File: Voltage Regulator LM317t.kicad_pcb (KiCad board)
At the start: 2 copper layers, 55.8 x 28 mm, 15 parts, among them J1 IN, J2 OUT, U1 LM317_TO-220

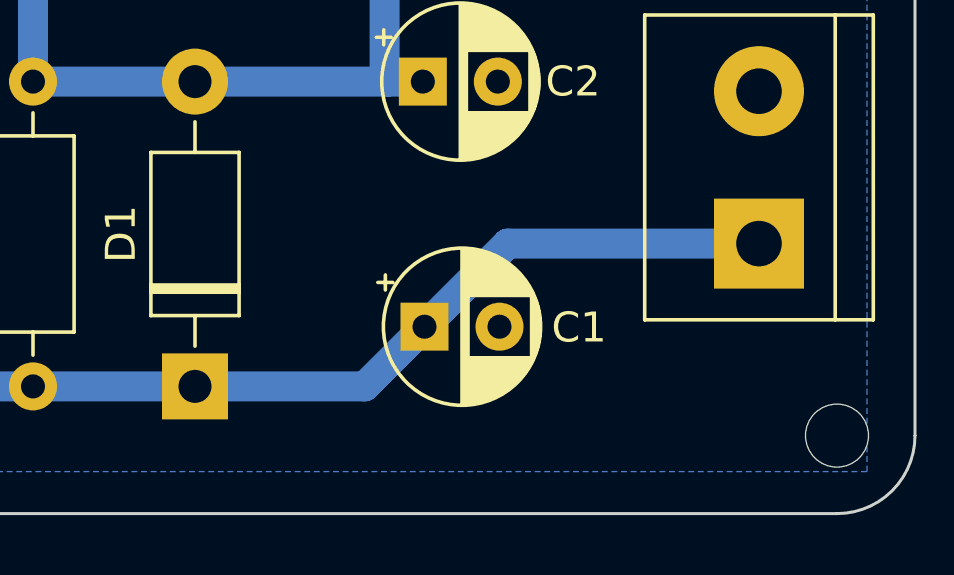
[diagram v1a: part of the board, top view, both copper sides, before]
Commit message: interactive bom
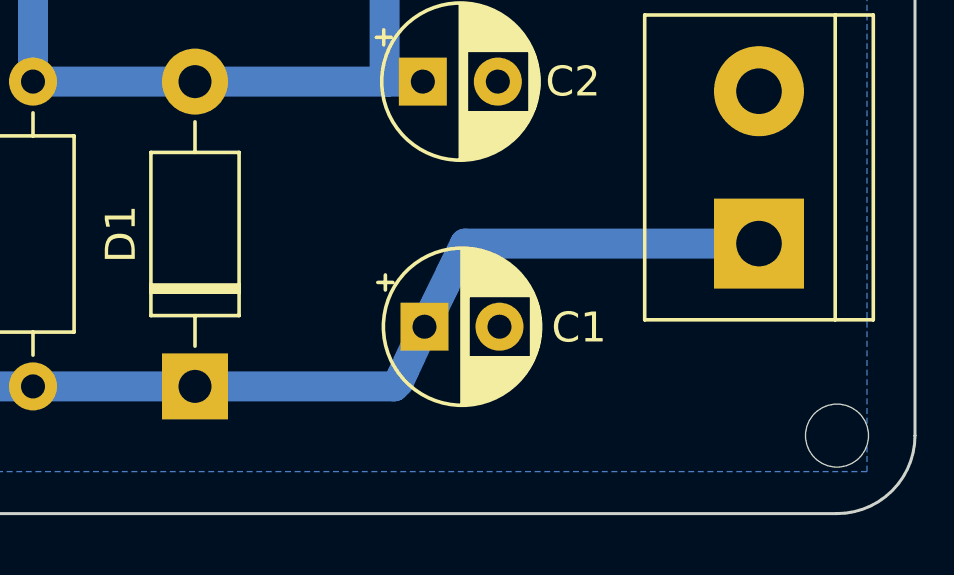
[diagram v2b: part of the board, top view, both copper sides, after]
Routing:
- net /OUTPUT: track 50.2 -> 51.2 mm
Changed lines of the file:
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@@
   )
   (paper "A4")
+  (title_block
+    (title "Voltage Regulator LM317T")
+    (date "2023-08-16")
+    (rev "1.0.0")
+  )
   (layers
-    (0 "F.Cu" signal)
-    (31 "B.Cu" signal)
+    (0 "F.Cu" power)
+    (31 "B.Cu" mixed)
     (32 "B.Adhes" user "B.Adhesive")
     (33 "F.Adhes" user "F.Adhesive")
@@
       (outputformat 1)
       (mirror false)
-      (drillshape 1)
+      (drillshape 0)
       (scaleselection 1)
-      (outputdirectory "")
+      (outputdirectory "./")
     )
   )
@@
     (property "ki_keywords" "mounting hole")
     (attr exclude_from_pos_files exclude_from_bom)
-    (fp_text reference "H1" (at -35.2 13.2) (layer "F.SilkS") hide
+    (fp_text reference "H1" (at 0 -4.2) (layer "F.SilkS") hide
         (effects (font (size 1 1) (thickness 0.15)))
     )
@@
         (effects (font (size 1 1) (thickness 0.15)))
     )
-    (fp_text user "${REFERENCE}" (at 2.54 -4.27) (layer "F.Fab")
+    (fp_text user "${REFERENCE}" (at 9 -0.05) (layer "F.Fab")
         (effects (font (size 1 1) (thickness 0.15)))
     )
@@
     (pad "3" thru_hole oval (at 5.08 0 180) (size 1.905 2) (drill 1.1) (layers "*.Cu" "*.Mask")
       (net 4 "/INPUT") (pinfunction "VI") (pintype "power_in"))
-    (model "${KIPRJMOD}/packages3D/TO-220-3_Vertical.wrl"
+    (model "${KICAD6_3DMODEL_DIR}/Package_TO_SOT_THT.3dshapes/TO-220-3_Vertical.wrl"
       (offset (xyz 0 0 0))
       (scale (xyz 1 1 1))
@@
         (effects (font (size 1 1) (thickness 0.15)))
     )
-    (fp_text value "Logo_Open_Hardware_Small" (at 0.75 0) (layer "B.Fab") hide
-        (effects (font (size 1 1) (thickness 0.15)) (justify mirror))
+    (fp_text value "Logo_Open_Hardware_Small" (at 0.75 0) (layer "F.SilkS") hide
+        (effects (font (size 1 1) (thickness 0.15)))
     )
     (fp_poly
@@
     (effects (font (size 1.5 1.5) (thickness 0.3) bold) (justify left bottom mirror))
   )
-  (segment (start 167.4 112.8) (end 159.02 112.8) (width 1) (layer "B.Cu") (net 1))
+  (dimension (type aligned) (layer "Dwgs.User")
+    (pts (xy 116.8 119.2) (xy 172.6 119.2))
+    (height 7.999999)
+    (gr_text "55.8000 mm" (at 144.7 126.049999) (layer "Dwgs.User")
+      (effects (font (size 1 1) (thickness 0.15)))
+    )
+    (format (prefix "") (suffix "") (units 3) (units_format 1) (precision 4))
+    (style (thickness 0.15) (arrow_length 1.27) (text_position_mode 0) (extension_height 0.58642) (extension_offset 0.5) keep_text_aligned)
+  )
+  (dimension (type aligned) (layer "Dwgs.User")
+    (pts (xy 170 121.8) (xy 170 93.8))
+    (height 11)
+    (gr_text "28.0000 mm" (at 179.85 107.8 90) (layer "Dwgs.User")
+      (effects (font (size 1 1) (thickness 0.15)))
+    )
+    (format (prefix "") (suffix "") (units 3) (units_format 1) (precision 4))
+    (style (thickness 0.15) (arrow_length 1.27) (text_position_mode 0) (extension_height 0.58642) (extension_offset 0.5) keep_text_aligned)
+  )
+  (dimension (type radial) (layer "Dwgs.User")
+    (pts (xy 119.4 119.2) (xy 117.561522 121.038478))
+    (leader_length 3.81)
+    (gr_text "R 2.6000 mm" (at 102.167445 123.732555) (layer "Dwgs.User")
+      (effects (font (size 1.5 1.5) (thickness 0.3)))
+    )
+    (format (prefix "R ") (suffix "") (units 3) (units_format 1) (precision 4))
+    (style (thickness 0.2) (arrow_length 1.27) (text_position_mode 0) (extension_offset 0.5) keep_text_aligned)
+  )
+  (segment (start 157.6 112.8) (end 156.25 115.57) (width 1) (layer "B.Cu") (net 1))
   (segment (start 140.6 117.56) (end 143.2 117.56) (width 1) (layer "B.Cu") (net 1))
   (segment (start 143.2 117.56) (end 148.6 117.56) (width 1) (layer "B.Cu") (net 1))
-  (segment (start 154.26 117.56) (end 156.25 115.57) (width 1) (layer "B.Cu") (net 1))
+  (segment (start 167.4 112.8) (end 157.6 112.8) (width 1) (layer "B.Cu") (net 1))
   (segment (start 140.66 117.5) (end 140.6 117.56) (width 1) (layer "B.Cu") (net 1))
+  (segment (start 155.4 117.4) (end 156.25 115.57) (width 1) (layer "B.Cu") (net 1))
   (segment (start 138 117.56) (end 140.6 117.56) (width 1) (layer "B.Cu") (net 1))
-  (segment (start 159.02 112.8) (end 156.25 115.57) (width 1) (layer "B.Cu") (net 1))
+  (segment (start 148.6 117.56) (end 155.24 117.56) (width 1) (layer "B.Cu") (net 1))
+  (segment (start 155.24 117.56) (end 155.4 117.4) (width 1) (layer "B.Cu") (net 1))
   (segment (start 140.66 98.75) (end 140.66 117.5) (width 1) (layer "B.Cu") (net 1))
-  (segment (start 148.6 117.56) (end 154.26 117.56) (width 1) (layer "B.Cu") (net 1))
   (segment (start 155 107.4) (end 156.194888 107.4) (width 1) (layer "B.Cu") (net 3))
   (segment (start 154.92 100) (end 154.92 107.32) (width 1) (layer "B.Cu") (net 3))
